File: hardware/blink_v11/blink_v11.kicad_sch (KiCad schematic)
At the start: 180 parts, among them J1 Conn_01x02, J14 Conn_02x16_Odd_Even, J15 Conn_01x01, J16 Conn_01x01, J5 Conn_01x06_Pin, J6 Conn_01x03, J7 Conn_01x06_Pin, J9 USB_C_Receptacle, Q1 AO3400A, Q2 AO3400A, Q3 2N7002, Q4 2N7002, Q5 2N7002, SW1 SW_SPDT, SW2 SW_Push_4PDT, SW3 SW_Push_4PDT, SW4 SW_Push_4PDT, U1 AMS1117-3.3, U10 TMP112AIDRLR, U11 MAX40200AUK, U12 MAX40200AUK, U13 AMS1117-3.3, U14 SN74LVC1G14DBV, U15 BQ29702DSER, U16 TPS63060, U3 M24C02-RMN, U4 STM32F405RGTx, U5 SN74LVC1G14DBV, U6 SN74LVC1G14DBV, U7 CH340C, U8 USBLC6-2P6, U9 MCP73832-2-OT, X1 GTXO-14V (2.048MHz), Y1 16MHz

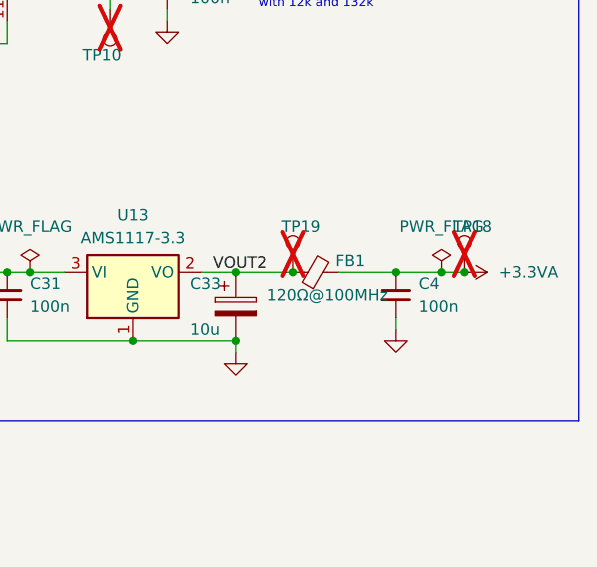
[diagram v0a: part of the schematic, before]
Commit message: clean up
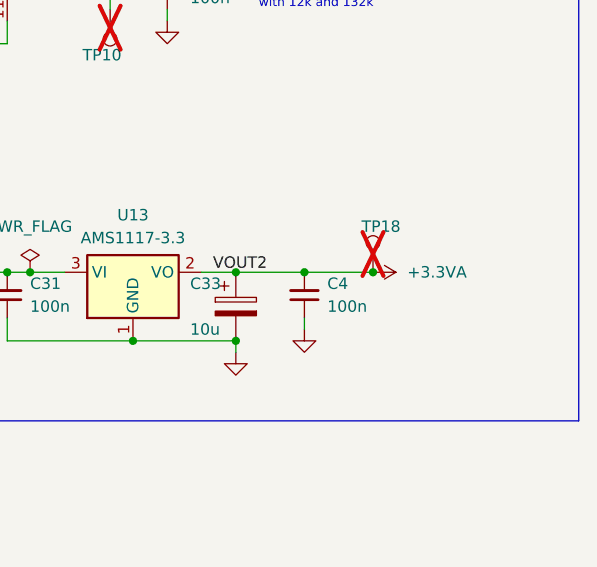
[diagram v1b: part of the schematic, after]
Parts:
- removed FB1: 120Ω@100MHz, Resistor_SMD:R_0603_1608Metric, symbol Device:FerriteBead_Small
- removed TP19: ~, TestPoint:TestPoint_THTPad_D1.5mm_Drill0.7mm, symbol Connector:TestPoint
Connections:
- net VOUT2 is gone; now on net +3.3VA: C33.1, U13.2 (VO)
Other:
- moved on the sheet: C4, TP18
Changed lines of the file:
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@@
   (junction (at 394.97 46.99) (diameter 0) (color 0 0 0 0)
   )
-  (junction (at 387.35 120.65) (diameter 0) (color 0 0 0 0)
-  )
   (junction (at 317.5 127) (diameter 0) (color 0 0 0 0)
   )
@@
   (junction (at 77.47 50.8) (diameter 0) (color 0 0 0 0)
   )
-  (junction (at 406.4 120.65) (diameter 0) (color 0 0 0 0)
+  (junction (at 396.24 120.65) (diameter 0) (color 0 0 0 0)
   )
   (junction (at 353.06 95.25) (diameter 0) (color 0 0 0 0)
@@
   (junction (at 123.19 233.68) (diameter 0) (color 0 0 0 0)
   )
-  (junction (at 398.78 120.65) (diameter 0) (color 0 0 0 0)
+  (junction (at 388.62 120.65) (diameter 0) (color 0 0 0 0)
   )
   (junction (at 224.79 36.83) (diameter 0) (color 0 0 0 0)
@@
   (junction (at 391.16 27.94) (diameter 0) (color 0 0 0 0)
   )
-  (junction (at 403.86 120.65) (diameter 0) (color 0 0 0 0)
-  )
   (junction (at 54.61 57.15) (diameter 0) (color 0 0 0 0)
   )
@@
     (stroke (width 0) (type default))
   )
-  (wire (pts (xy 398.78 125.73) (xy 398.78 127))
+  (wire (pts (xy 388.62 125.73) (xy 388.62 127))
     (stroke (width 0) (type default))
   )
@@
     (stroke (width 0) (type default))
   )
-  (wire (pts (xy 392.43 120.65) (xy 398.78 120.65))
-    (stroke (width 0) (type default))
-  )
   (wire (pts (xy 311.15 26.67) (xy 311.15 33.02))
     (stroke (width 0) (type default))
@@
     (stroke (width 0) (type default))
   )
-  (wire (pts (xy 403.86 120.65) (xy 406.4 120.65))
+  (wire (pts (xy 388.62 120.65) (xy 396.24 120.65))
     (stroke (width 0) (type default))
   )
@@
     (stroke (width 0) (type default))
   )
-  (wire (pts (xy 398.78 120.65) (xy 403.86 120.65))
-    (stroke (width 0) (type default))
-  )
   (wire (pts (xy 161.29 162.56) (xy 166.37 162.56))
     (stroke (width 0) (type default))
@@
     (stroke (width 0) (type default))
   )
-  (wire (pts (xy 381 120.65) (xy 387.35 120.65))
+  (wire (pts (xy 381 120.65) (xy 388.62 120.65))
     (stroke (width 0) (type default))
   )
@@
     )
   )
-  (symbol (lib_id "power:GND") (at 398.78 127 0) (unit 1)
+  (symbol (lib_id "power:GND") (at 388.62 127 0) (unit 1)
     (in_bom yes) (on_board yes) (dnp no)
-    (property "Reference" "#PWR07" (at 398.78 133.35 0)
+    (property "Reference" "#PWR07" (at 388.62 133.35 0)
       (effects (font (size 1.27 1.27)) hide)
     )
-    (property "Value" "GND" (at 398.78 132.08 0)
+    (property "Value" "GND" (at 388.62 132.08 0)
       (effects (font (size 1.27 1.27)) hide)
     )
-    (property "Footprint" "" (at 398.78 127 0)
+    (property "Footprint" "" (at 388.62 127 0)
       (effects (font (size 1.27 1.27)) hide)
     )
-    (property "Datasheet" "" (at 398.78 127 0)
+    (property "Datasheet" "" (at 388.62 127 0)
       (effects (font (size 1.27 1.27)) hide)
     )
@@
     )
   )
-  (symbol (lib_id "Device:C_Small") (at 398.78 123.19 180) (unit 1)
+  (symbol (lib_id "Device:C_Small") (at 388.62 123.19 180) (unit 1)
     (in_bom yes) (on_board yes) (dnp no) (fields_autoplaced)
-    (property "Reference" "C4" (at 401.32 121.9136 0)
+    (property "Reference" "C4" (at 391.16 121.9136 0)
       (effects (font (size 1.27 1.27)) (justify right))
     )
-    (property "Value" "100n" (at 401.32 124.4536 0)
+    (property "Value" "100n" (at 391.16 124.4536 0)
       (effects (font (size 1.27 1.27)) (justify right))
     )
-    (property "Footprint" "Capacitor_SMD:C_0603_1608Metric" (at 398.78 123.19 0)
+    (property "Footprint" "Capacitor_SMD:C_0603_1608Metric" (at 388.62 123.19 0)
       (effects (font (size 1.27 1.27)) hide)
     )
-    (property "Datasheet" "~" (at 398.78 123.19 0)
+    (property "Datasheet" "~" (at 388.62 123.19 0)
       (effects (font (size 1.27 1.27)) hide)
     )
-    (property "LCSC" "" (at 398.78 123.19 0)
+    (property "LCSC" "" (at 388.62 123.19 0)
       (effects (font (size 1.27 1.27)) hide)
     )
-    (property "JLCPCB Part #" "C14663" (at 398.78 123.19 0)
+    (property "JLCPCB Part #" "C14663" (at 388.62 123.19 0)
       (effects (font (size 1.27 1.27)) hide)
     )
@@
     )
   )
-  (symbol (lib_id "power:PWR_FLAG") (at 403.86 120.65 0) (unit 1)
-    (in_bom yes) (on_board yes) (dnp no) (fields_autoplaced)
-    (property "Reference" "#FLG02" (at 403.86 118.745 0)
-      (effects (font (size 1.27 1.27)) hide)
-    )
-    (property "Value" "PWR_FLAG" (at 403.86 115.57 0)
-      (effects (font (size 1.27 1.27)))
-    )
-    (property "Footprint" "" (at 403.86 120.65 0)
-      (effects (font (size 1.27 1.27)) hide)
-    )
-    (property "Datasheet" "~" (at 403.86 120.65 0)
-      (effects (font (size 1.27 1.27)) hide)
-    )
-    (pin "1")
-    (instances
-      (project "blink_v11"
-        (path "/bd4d3b9a-07c1-4a53-9c94-2893f3e869d4"
-          (reference "#FLG02") (unit 1)
-        )
-      )
-    )
-  )
   (symbol (lib_id "Device:C_Small") (at 20.32 96.52 180) (unit 1)
     (in_bom yes) (on_board yes) (dnp no) (fields_autoplaced)
@@
     )
   )
-  (symbol (lib_id "Connector:TestPoint") (at 406.4 120.65 0) (unit 1)
+  (symbol (lib_id "Connector:TestPoint") (at 396.24 120.65 0) (unit 1)
     (in_bom no) (on_board yes) (dnp yes)
-    (property "Reference" "TP18" (at 405.13 115.57 0)
+    (property "Reference" "TP18" (at 394.97 115.57 0)
       (effects (font (size 1.27 1.27)) (justify left))
     )
-    (property "Value" "~" (at 405.13 114.3 0)
+    (property "Value" "~" (at 394.97 114.3 0)
       (effects (font (size 1.27 1.27)) (justify left))
     )
-    (property "Footprint" "TestPoint:TestPoint_THTPad_D1.5mm_Drill0.7mm" (at 411.48 120.65 0)
+    (property "Footprint" "TestPoint:TestPoint_THTPad_D1.5mm_Drill0.7mm" (at 401.32 120.65 0)
       (effects (font (size 1.27 1.27)) hide)
     )
-    (property "Datasheet" "~" (at 411.48 120.65 0)
+    (property "Datasheet" "~" (at 401.32 120.65 0)
       (effects (font (size 1.27 1.27)) hide)
     )
@@
     )
   )
-  (symbol (lib_id "power:+3.3VA") (at 406.4 120.65 270) (unit 1)
+  (symbol (lib_id "power:+3.3VA") (at 396.24 120.65 270) (unit 1)
     (in_bom yes) (on_board yes) (dnp no) (fields_autoplaced)
-    (property "Reference" "#PWR09" (at 402.59 120.65 0)
+    (property "Reference" "#PWR09" (at 392.43 120.65 0)
       (effects (font (size 1.27 1.27)) hide)
     )
-    (property "Value" "+3.3VA" (at 410.21 120.65 90)
+    (property "Value" "+3.3VA" (at 400.05 120.65 90)
       (effects (font (size 1.27 1.27)) (justify left))
     )
-    (property "Footprint" "" (at 406.4 120.65 0)
+    (property "Footprint" "" (at 396.24 120.65 0)
       (effects (font (size 1.27 1.27)) hide)
     )
-    (property "Datasheet" "" (at 406.4 120.65 0)
+    (property "Datasheet" "" (at 396.24 120.65 0)
       (effects (font (size 1.27 1.27)) hide)
     )
@@
     )
   )
-  (symbol (lib_id "Device:FerriteBead_Small") (at 389.89 120.65 90) (unit 1)
-    (in_bom yes) (on_board yes) (dnp no)
-    (property "Reference" "FB1" (at 393.7 119.38 90)
-      (effects (font (size 1.27 1.27)))
-    )
-    (property "Value" "120Ω@100MHz " (at 391.16 123.19 90)
-      (effects (font (size 1.27 1.27)))
-    )
-    (property "Footprint" "Resistor_SMD:R_0603_1608Metric" (at 389.89 122.428 90)
-      (effects (font (size 1.27 1.27)) hide)
-    )
-    (property "Datasheet" "~" (at 389.89 120.65 0)
-      (effects (font (size 1.27 1.27)) hide)
-    )
-    (property "LCSC" "" (at 389.89 120.65 0)
-      (effects (font (size 1.27 1.27)) hide)
-    )
-    (property "JLCPCB Part #" "C127301" (at 389.89 120.65 0)
-      (effects (font (size 1.27 1.27)) hide)
-    )
-    (pin "1")
-    (pin "2")
-    (instances
-      (project "blink_v11"
-        (path "/bd4d3b9a-07c1-4a53-9c94-2893f3e869d4"
-          (reference "FB1") (unit 1)
-        )
-      )
-    )
-  )
   (symbol (lib_id "Device:C_Polarized") (at 317.5 123.19 0) (unit 1)
     (in_bom yes) (on_board yes) (dnp no)
@@
         )
       )
-    )
-  )
-  (symbol (lib_id "Connector:TestPoint") (at 387.35 120.65 0) (unit 1)
-    (in_bom no) (on_board yes) (dnp yes)
-    (property "Reference" "TP19" (at 386.08 115.57 0)
-      (effects (font (size 1.27 1.27)) (justify left))
-    )
-    (property "Value" "~" (at 386.08 114.3 0)
-      (effects (font (size 1.27 1.27)) (justify left))
-    )
-    (property "Footprint" "TestPoint:TestPoint_THTPad_D1.5mm_Drill0.7mm" (at 392.43 120.65 0)
-      (effects (font (size 1.27 1.27)) hide)
-    )
-    (property "Datasheet" "~" (at 392.43 120.65 0)
-      (effects (font (size 1.27 1.27)) hide)
-    )
-    (pin "1")
-    (instances
-      (project "blink_v11"
-        (path "/bd4d3b9a-07c1-4a53-9c94-2893f3e869d4"
-          (reference "TP19") (unit 1)
-        )
-      )
